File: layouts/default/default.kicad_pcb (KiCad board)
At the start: 2 copper layers, 47 parts

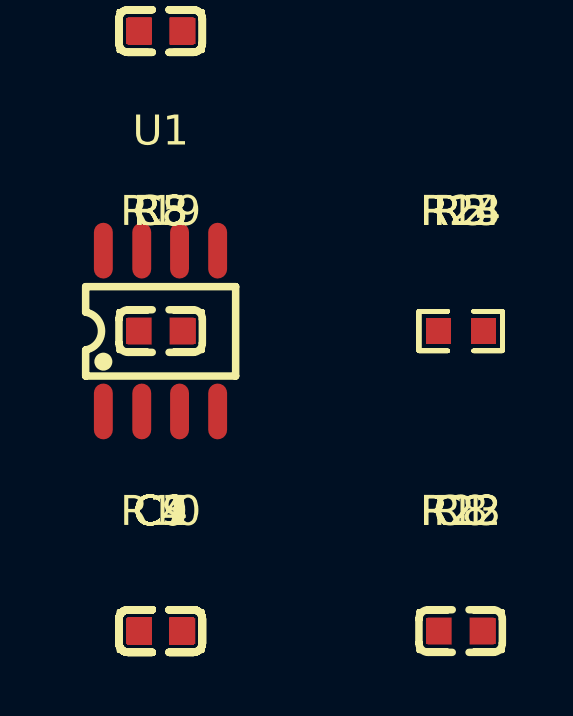
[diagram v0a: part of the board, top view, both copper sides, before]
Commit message: summing stage and bug fix
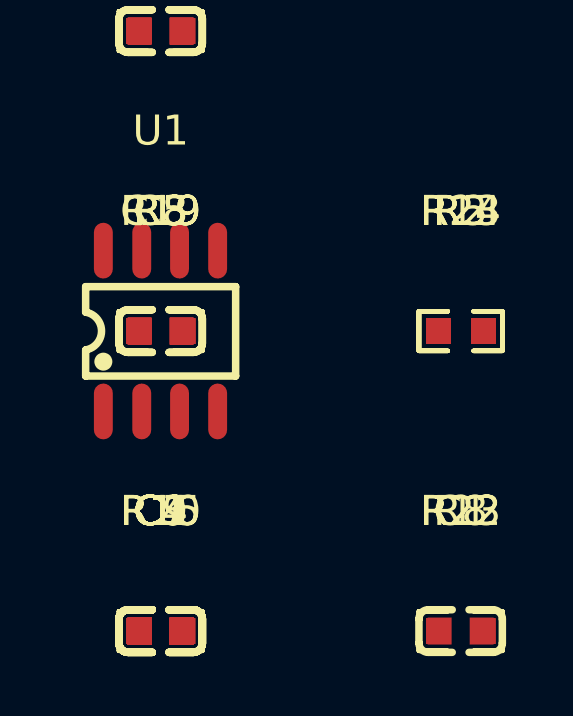
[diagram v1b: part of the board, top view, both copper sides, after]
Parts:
- added C19: 100nF ±10% 50V X7R, atopile:C0603-bd72f6, F.Cu at (0.00, -10.0)
- added R15: 10kΩ ±1% 100mW, atopile:R0603-ebcab9, F.Cu at (0.00, 0.00)
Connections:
- C11 pad 2: net-1 -> net-6
- C12 pad 2: net -> net-4
- C13 pad 1: net-4 -> net-5
- C17 pad 2: cathode -> net-1
- C18 pad 1: anode -> cathode-1
- C18 pad 2: net -> net-4
- C2 pad 1: resistors_ifs[1] -> P1INplus
- C3 pad 1: VOUT -> gnd-1
- C5 pad 2: cathode-1 -> cathode
- C6 pad 1: cathode-2 -> VCCplus
- C7 pad 1: net-5 -> net
- C7 pad 2: resistors_ifs[1] -> P1INplus
- C9 pad 1: resistors_ifs[1] -> P1INplus
- D1 pad 1: cathode-1 -> cathode
- D2 pad 1: cathode-2 -> VCCplus
- D2 pad 2: cathode-1 -> cathode
- R1 pad 1: resistors_ifs[1] -> P1INplus
- R12 pad 2: net-4 -> net-5
- R14 pad 1: resistors_ifs[1] -> P1INplus
- R17 pad 1: resistors_ifs[1]-1 -> resistors_ifs[1]
- R2 pad 2: resistors_ifs[1] -> P1INplus
- R20 pad 1: cathode -> net-1
- R20 pad 2: anode -> cathode-1
- R21 pad 1: net -> net-4
- R22 pad 2: resistors_ifs[1] -> P1INplus
- R23 pad 1: resistors_ifs[1]-1 -> resistors_ifs[1]
- R23 pad 2: resistors_ifs[1] -> P1INplus
- R3 pad 1: input_dc_bias_r-net-1 -> input_dc_bias_r-net
- R3 pad 2: input_dc_bias_r-net -> input_dc_bias_r-net-1
- R4 pad 2: net-5 -> net
- R8 pad 2: resistors_ifs[1] -> P1INplus
- R9 pad 1: net-1 -> net-6
- R9 pad 2: resistors_ifs[1] -> P1INplus
- U1 pad 5: VOUT -> gnd-1
- U2 pad 1: resistors_ifs[1] -> P1INplus
- U2 pad 3: resistors_ifs[1] -> P1INplus
- U3 pad 4: tone_opamps-gnd -> gnd-1
- U4 pad 2: anode -> cathode-1
- U5 pad 1: cathode -> cathode-1
